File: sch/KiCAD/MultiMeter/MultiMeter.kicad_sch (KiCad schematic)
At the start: 20 parts, among them J1 Conn_01x02_Male, J2 Conn_01x02_Male, J3 Conn_01x03_Male, J4 Conn_01x03_Male, J5 Conn_01x02_Female, J6 Conn_01x15, J7 Conn_01x15

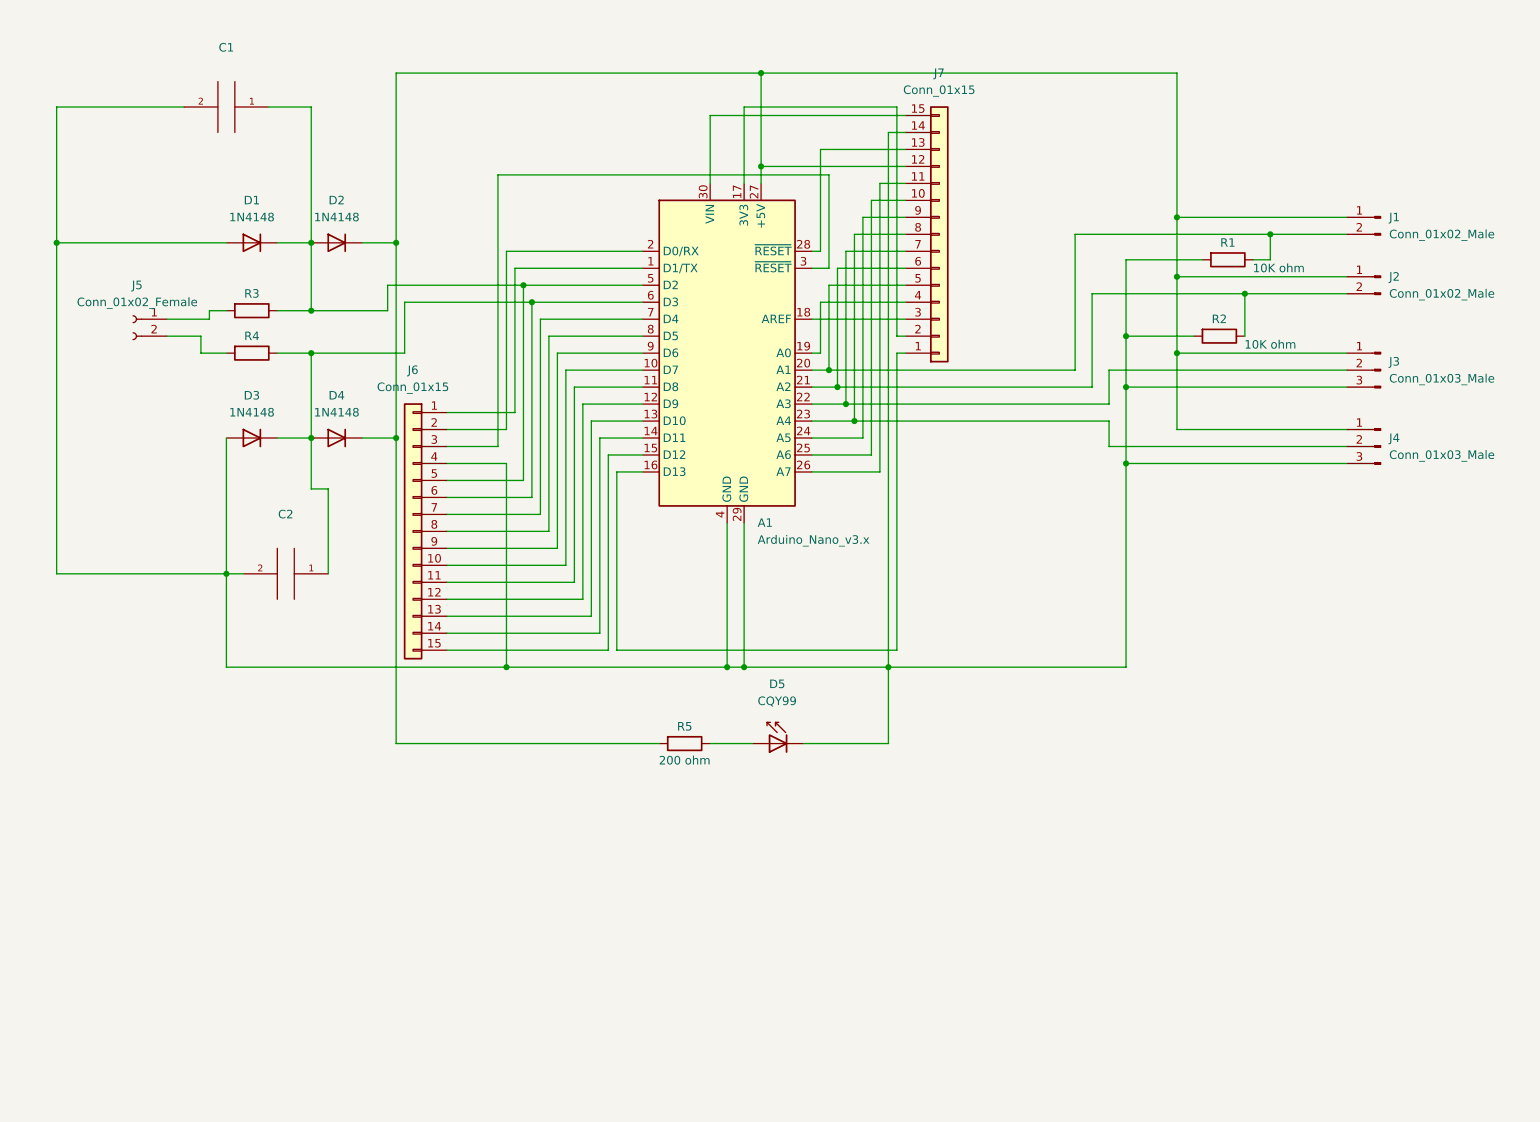
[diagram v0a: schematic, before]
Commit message: 基板修正
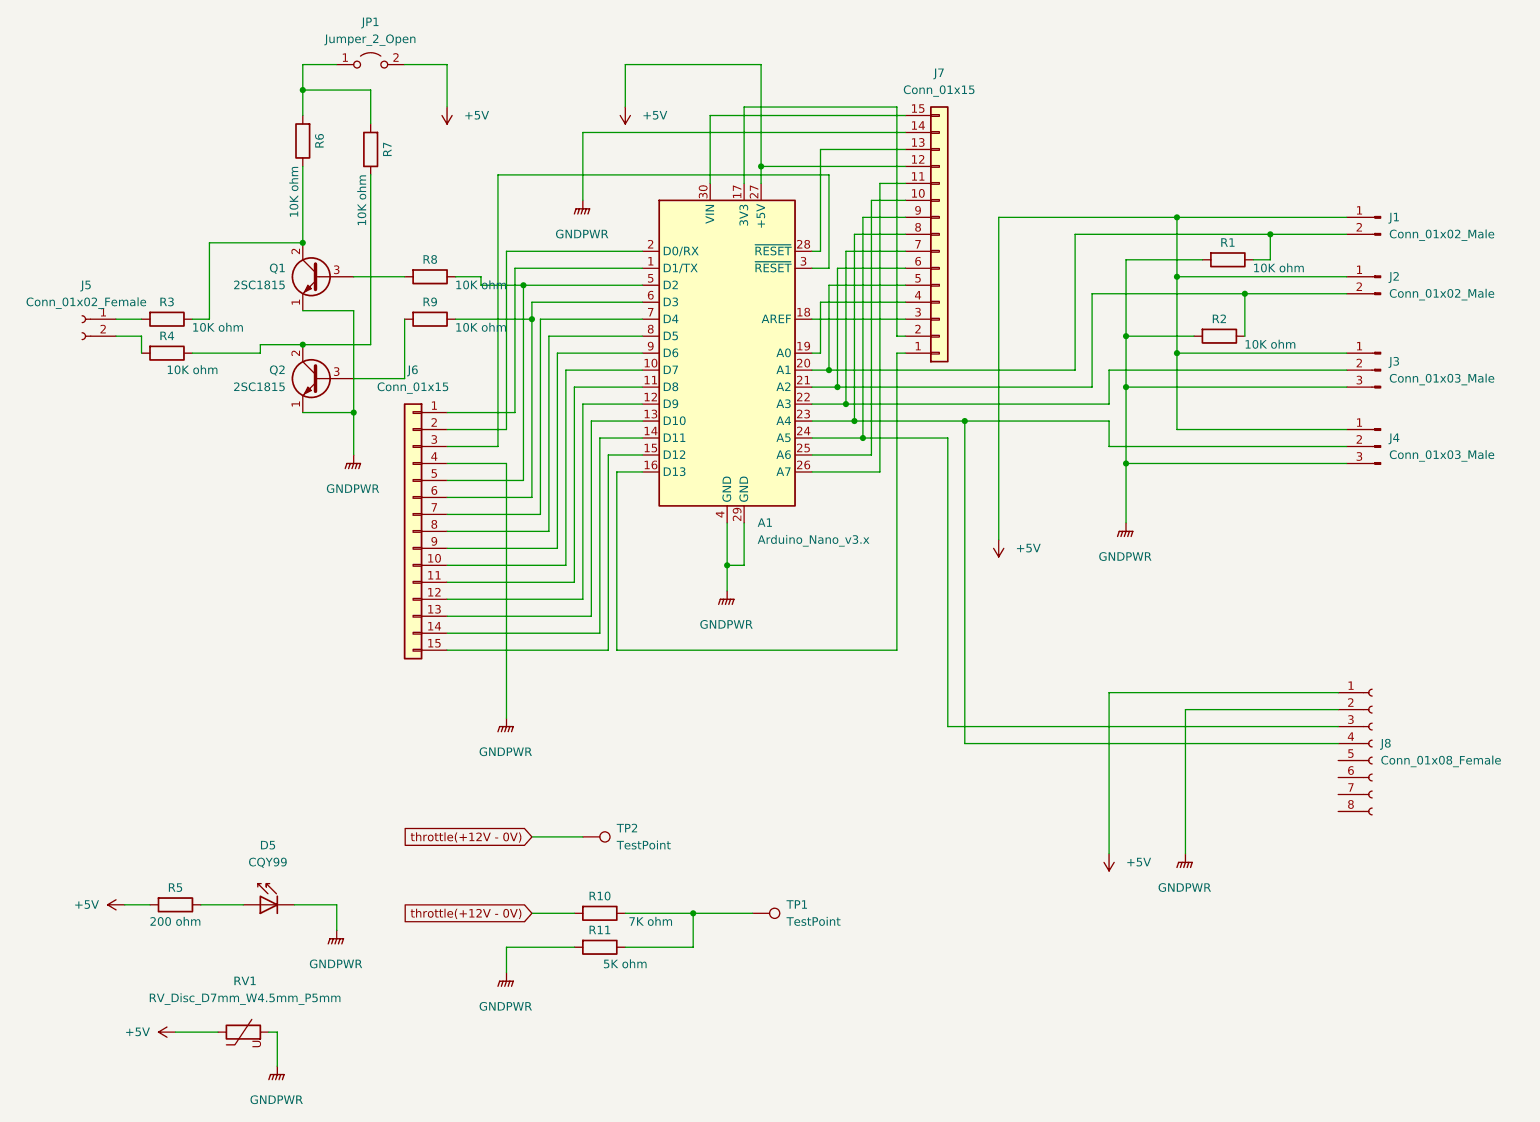
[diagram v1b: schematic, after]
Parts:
- removed C1, C2: (no value), Capacitor_THT:C_Rect_L4.6mm_W2.0mm_P2.50mm_MKS02_FKP02, symbol pspice:C
- removed D1, D2, D3, D4: 1N4148, Diode_THT:D_DO-35_SOD27_P7.62mm_Horizontal, symbol Diode:1N4148
- added J8: Conn_01x08_Female, Connector_JST:JST_XH_B8B-XH-A_1x08_P2.50mm_Vertical, symbol Connector:Conn_01x08_Female
- added JP1: Jumper_2_Open, Connector_PinHeader_2.54mm:PinHeader_1x02_P2.54mm_Vertical, symbol Jumper:Jumper_2_Open
- added Q1, Q2: 2SC1815, Package_TO_SOT_THT:TO-92_Inline, symbol Transistor_BJT:2SC1815
- added R10: 7K ohm, Resistor_THT:R_Axial_DIN0204_L3.6mm_D1.6mm_P7.62mm_Horizontal, symbol Device:R
- added R11: 5K ohm, Resistor_THT:R_Axial_DIN0204_L3.6mm_D1.6mm_P7.62mm_Horizontal, symbol Device:R
- added R6, R7, R8, R9: 10K ohm, Resistor_THT:R_Axial_DIN0204_L3.6mm_D1.6mm_P7.62mm_Horizontal, symbol Device:R
- added RV1: RV_Disc_D7mm_W4.5mm_P5mm, Varistor:RV_Disc_D7mm_W4.5mm_P5mm, symbol Device:Varistor
- added TP1, TP2: TestPoint, MountingHole:MountingHole_2.2mm_M2_DIN965_Pad, symbol Connector:TestPoint
- J1, J2: footprint Connector_Molex:Molex_SPOX_5267-02A_1x02_P2.50mm_Vertical -> Connector_Molex:Molex_SPOX_5268-02A_1x02_P2.50mm_Horizontal
- J3, J4: footprint Connector_Molex:Molex_SPOX_5267-03A_1x03_P2.50mm_Vertical -> Connector_Molex:Molex_SPOX_5268-03A_1x03_P2.50mm_Horizontal
- R3, R4: value (none) -> 10K ohm
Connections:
- net at A1.6 (D3), J6.6 (Pin_6): now also R9.1; no longer R4.1
- net +5V: now reaches A1.27 (+5V), J1.1 (Pin_1), J2.1 (Pin_1), J3.1 (Pin_1), J4.1 (Pin_1), J7.12 (Pin_12), R5.2
- net +5V: now also J8.1 (Pin_1), JP1.2 (B), RV1.1
- net at A1.5 (D2), J6.5 (Pin_5): now also R8.1; no longer R3.1
- net GNDPWR: now reaches A1.29 (GND), A1.4 (GND), D5.1 (K), J3.3 (Pin_3), J4.3 (Pin_3), J6.4 (Pin_4), J7.14 (Pin_14), R1.2, R2.2
- net GNDPWR: now also J8.2 (Pin_2), Q1.1 (E), Q2.1 (E), R11.2, RV1.2
- net at A1.23 (A4), J4.2 (Pin_2), J7.8 (Pin_8): now also J8.4 (Pin_4)
- net at A1.24 (A5), J7.9 (Pin_9): now also J8.3 (Pin_3)
- new net: Q2.2 (C), R4.1, R7.1
- new net: R10.1, R11.1, TP1.1
- new net: JP1.1 (A), R6.2, R7.2
- new net: Q1.2 (C), R3.1, R6.1
- new net: Q1.3 (B), R8.2
- new net: Q2.3 (B), R9.2
- new net throttle(+12V - 0V): R10.2, TP2.1
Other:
- moved on the sheet: D5, J5, R3, R4, R5
